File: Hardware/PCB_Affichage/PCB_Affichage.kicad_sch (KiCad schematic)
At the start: 0 parts

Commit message: finalisation PCB Rack
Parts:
- added C1, C5: 100n, Capacitor_SMD:C_0603_1608Metric_Pad1.08x0.95mm_HandSolder, symbol Device:C
- added C2: 1u, Capacitor_SMD:C_0201_0603Metric_Pad0.64x0.40mm_HandSolder, symbol Device:C
- added C3: 100u, Capacitor:Wurth-100u, symbol Device:C_Polarized
- added D1: TVS, Diode_SMD:Nexperia_DSN1608-2_1.6x0.8mm, symbol Diode:PTVS7V5Z1USK
- added D2: LED, LED_SMD:LED_0603_1608Metric_Pad1.05x0.95mm_HandSolder, symbol Device:LED
- added J1: Conn_01x03, Conn_Alim:Conn_Secteur, symbol Connector_Generic:Conn_01x03
- added R3: 2k5, Resistor_SMD:R_0603_1608Metric_Pad0.98x0.95mm_HandSolder, symbol Device:R
- added R5, R6: 2k2, Resistor_SMD:R_0603_1608Metric_Pad0.98x0.95mm_HandSolder, symbol Device:R
- added SW1: SW_SPST, Switch:Wurth_2pin_P5.0mm, symbol Switch:SW_SPST
- added U1: ~, ESP32_C3_SuperMini:C3_SuperMini, symbol ESP32_C3_SuperMini:SuperMini_1
- added U2: ~, AC_DC_module:MP-LDE06-20B05, symbol AC-DC-5V:U_1
- added U3: PCF8575DBR, Package_SO:SSOP-24_5.3x8.2mm_P0.65mm, symbol Interface_Expansion:PCF8575DBR
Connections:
- new net: D2.2 (A), R3.2
- new net +5V: C1.1, C2.1, C3.1, C5.2, D1.1 (K), R3.1, R5.1, R6.1, U1.8 (5V), U2.4 (DC+), U3.24 (VCC)
- new net Earth: J1.3 (Pin_3)
- new net GND: C1.2, C2.2, C3.2, C5.1, D1.2 (A), D2.1 (K), U1.7 (GND), U2.3 (DC-), U3.12 (GND), U3.2 (A1), U3.21 (A0), U3.3 (A2)
- new net INA1_1: U3.4 (P0)
- new net INA1_2: U3.5 (P1)
- new net INA2_1: U3.6 (P2)
- new net INA2_2: U3.7 (P3)
- new net INA3_1: U3.8 (P4)
- new net INA3_2: U3.9 (P5)
- new net INA4_1: U3.10 (P6)
- new net INA4_2: U3.11 (P7)
- new net INA5_1: U3.13 (P10)
- new net INA5_2: U3.14 (P11)
- new net INA6_1: U3.15 (P12)
- new net INA6_2: U3.16 (P13)
- new net LINE: SW1.1 (A), U2.2 (L)
- new net NEUT: J1.2 (Pin_2), U2.1 (N)
- new net On/Off: U1.14 (GPIO10)
- new net Phase: J1.1 (Pin_1), SW1.2 (B)
- new net Px: U1.9 (GPIO5)
- new net SCL: R5.2, U1.13 (GPIO9), U3.22 (SCL)
- new net SDA: R6.2, U1.12 (GPIO8), U3.23 (SDA)
- no-connect marks 0 -> 15
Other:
- note added: "Alimentation (230VAC)"
- note added: "Commande Neopixels"
- note added: "ESP32-C3"
- note added: "PSU AC/DC Input : 230V AC Output : 5V DC"

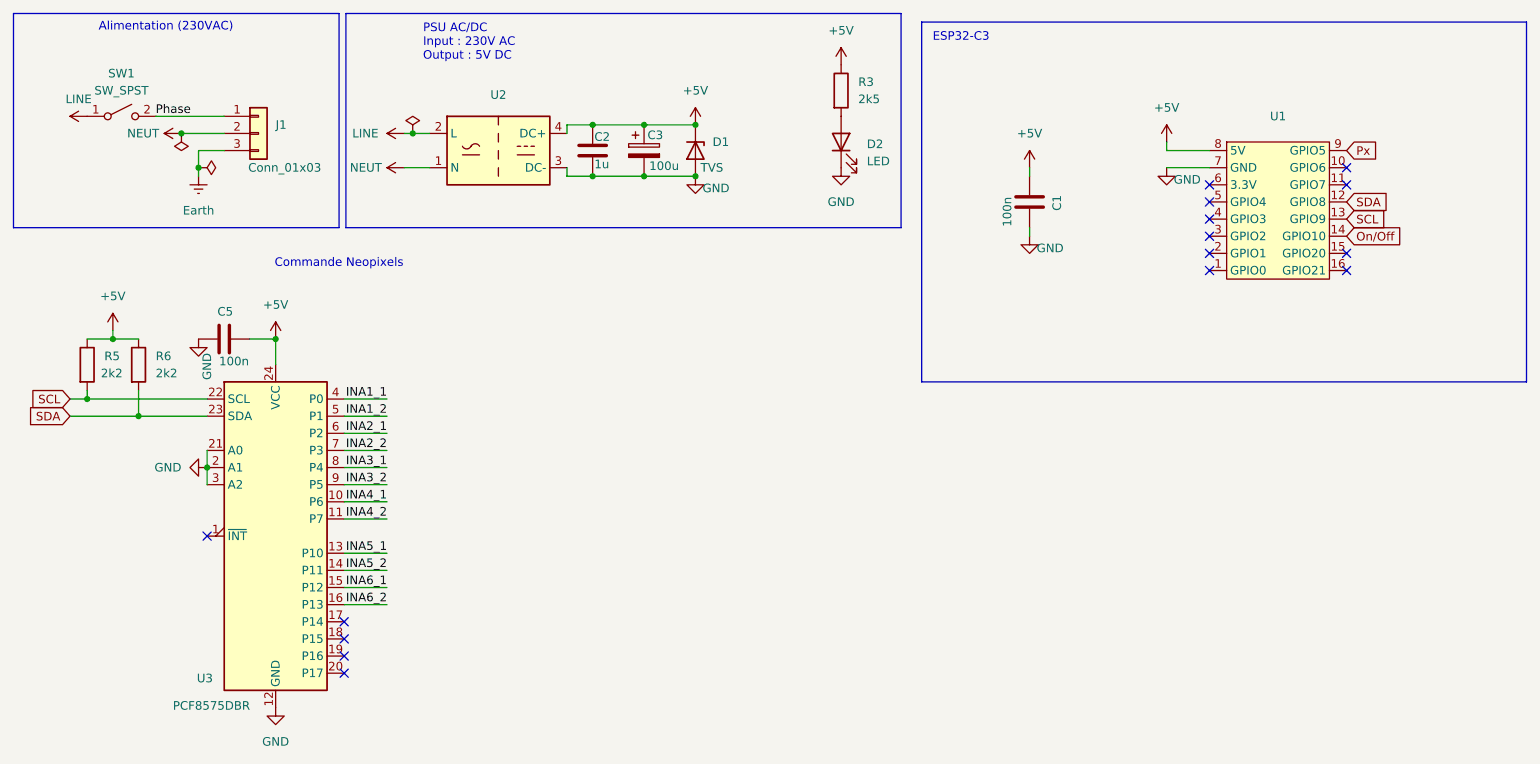
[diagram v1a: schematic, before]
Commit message: finalisation PCB affichage
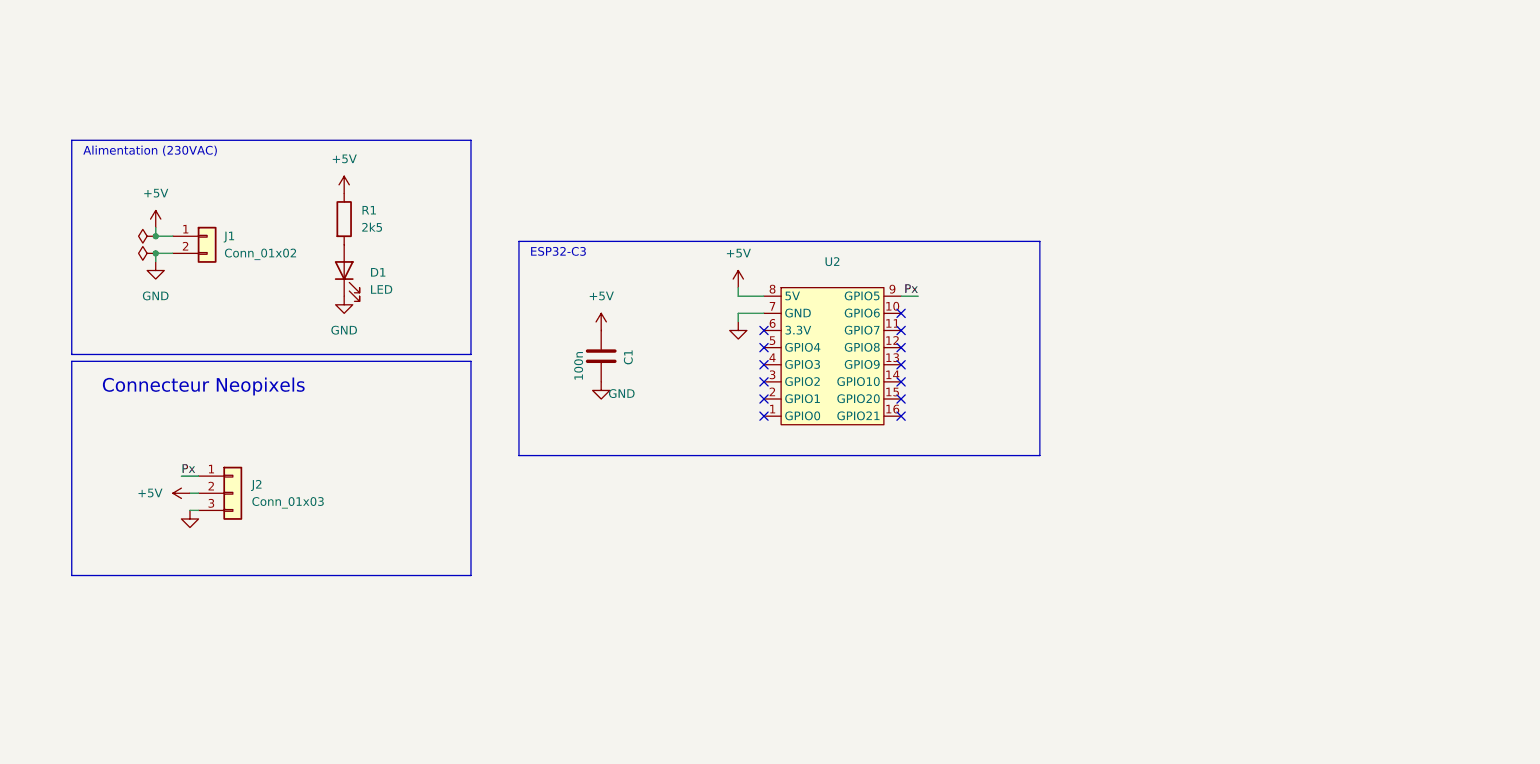
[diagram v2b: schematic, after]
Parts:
- removed C2: 1u, Capacitor_SMD:C_0201_0603Metric_Pad0.64x0.40mm_HandSolder, symbol Device:C
- removed C3: 100u, Capacitor:Wurth-100u, symbol Device:C_Polarized
- removed C5: 100n, Capacitor_SMD:C_0603_1608Metric_Pad1.08x0.95mm_HandSolder, symbol Device:C
- removed D1: TVS, Diode_SMD:Nexperia_DSN1608-2_1.6x0.8mm, symbol Diode:PTVS7V5Z1USK
- removed J1: Conn_01x03, Conn_Alim:Conn_Secteur, symbol Connector_Generic:Conn_01x03
- removed R5, R6: 2k2, Resistor_SMD:R_0603_1608Metric_Pad0.98x0.95mm_HandSolder, symbol Device:R
- removed SW1: SW_SPST, Switch:Wurth_2pin_P5.0mm, symbol Switch:SW_SPST
- removed U1: ~, ESP32_C3_SuperMini:C3_SuperMini, symbol ESP32_C3_SuperMini:SuperMini_1
- removed U2: ~, AC_DC_module:MP-LDE06-20B05, symbol AC-DC-5V:U_1
- removed U3: PCF8575DBR, Package_SO:SSOP-24_5.3x8.2mm_P0.65mm, symbol Interface_Expansion:PCF8575DBR
- added J1: Conn_01x02, Connector_AMASS:AMASS_XT30U-F_1x02_P5.0mm_Vertical, symbol Connector_Generic:Conn_01x02
- added J2: Conn_01x03, Conn:MR30_F, symbol Connector_Generic:Conn_01x03
- added U2: ~, ESP32_SuperMini:SuperMini SMT, symbol ESP32_C3:SuperMini_1
- renumbered D2 to D1, R3 to R1
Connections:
- net +5V: now also J1.1 (Pin_1), J2.2 (Pin_2), U2.8 (5V)
- net GND: now also J1.2 (Pin_2), J2.3 (Pin_3), U2.7 (GND)
- net Px: now also J2.1 (Pin_1), U2.9 (GPIO5)
- no-connect marks 15 -> 13
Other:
- note added: "Connecteur Neopixels"
- note removed: "Commande Neopixels"
- note removed: "PSU AC/DC Input : 230V AC Output : 5V DC"
- moved on the sheet: C1, D1, R1
